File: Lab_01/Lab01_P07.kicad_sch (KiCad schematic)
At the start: 7 parts

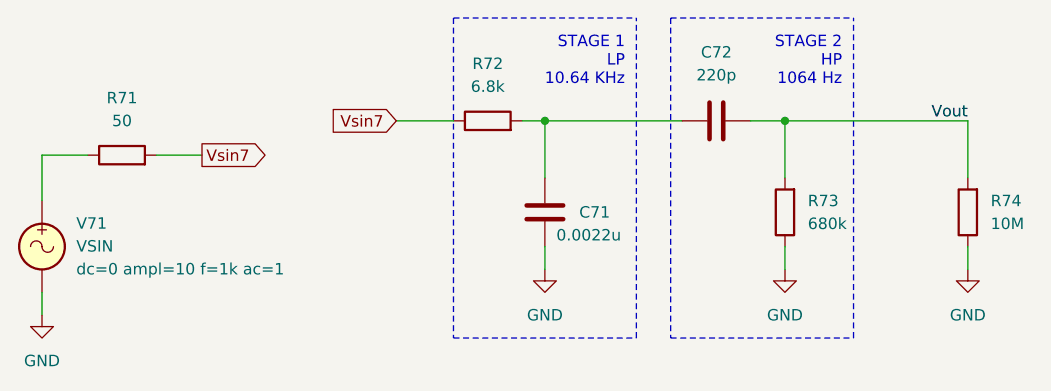
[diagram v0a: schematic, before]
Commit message: Edit up to Question 9
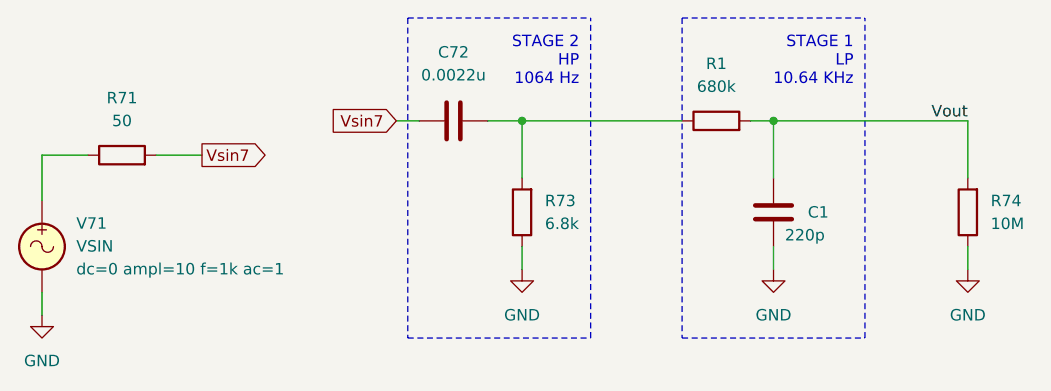
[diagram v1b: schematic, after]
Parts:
- removed C71: 0.0022u, symbol Device:C
- removed R72: 6.8k, symbol Device:R
- added C1: 220p, symbol Device:C
- added R1: 680k, symbol Device:R
- C72: value 220p -> 0.0022u
- R73: value 680k -> 6.8k
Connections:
- net GND: now also C1.2
- net Vout: now also C1.1, R1.2; no longer C72.2, R73.2
- net Vsin7: now also C72.1
- new net: C72.2, R1.1, R73.2
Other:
- moved on the sheet: C72, R73
